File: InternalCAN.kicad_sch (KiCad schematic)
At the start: 7 parts, among them J11 CAN_1, U4 ISO1044BD, U5 CDSOT23-T24CAN

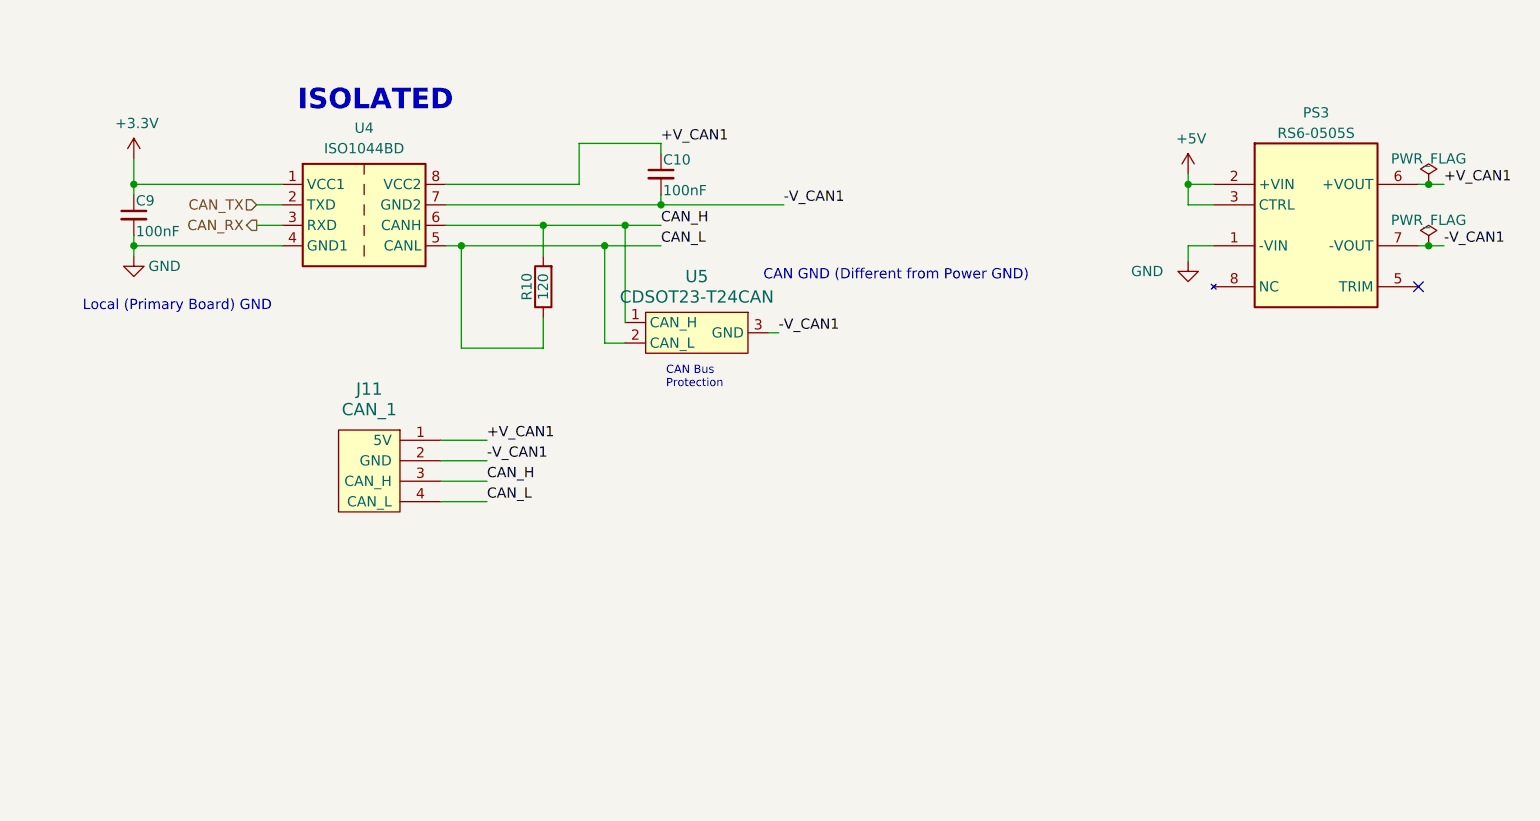
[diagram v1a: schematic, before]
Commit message: a
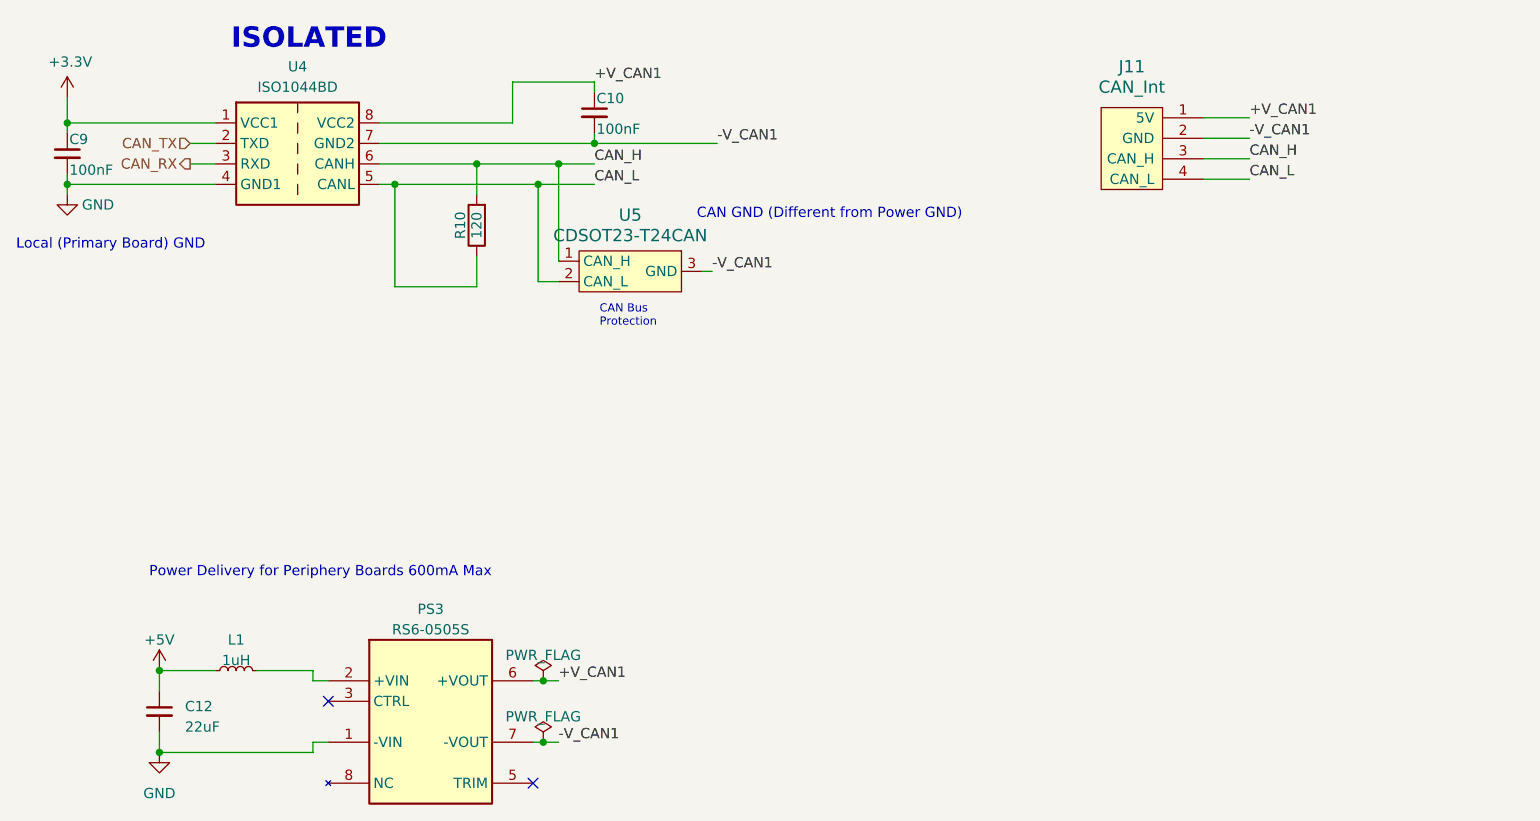
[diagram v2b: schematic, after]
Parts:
- added C12: 22uF, Capacitor_SMD:C_0805_2012Metric, symbol Device:C_Small
- added L1: 1uH, Inductor_SMD:L_0805_2012Metric, symbol Device:L_Small
- J11: value CAN_1 -> CAN_Int
- PS3: footprint RS60505S -> UTSVT_Power:RS60505S
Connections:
- net +5V: now also C12.1, L1.1; no longer PS3.2 (+VIN), PS3.3 (CTRL)
- net GND: now also C12.2
- new net: L1.2, PS3.2 (+VIN)
- no-connect marks 1 -> 2
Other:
- note added: "Power Delivery for Periphery Boards 600mA Max"
- moved on the sheet: C10, C9, J11, PS3, R10, U4, U5

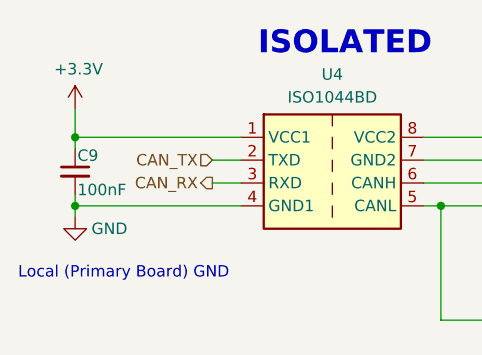
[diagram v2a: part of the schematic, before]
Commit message: updated pin assignments
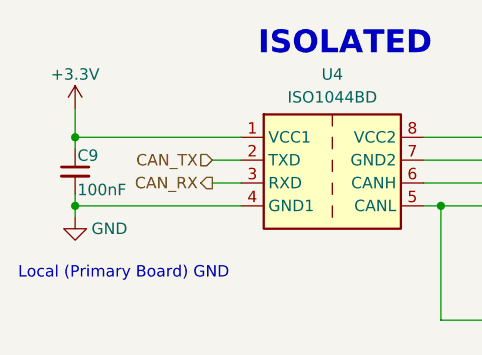
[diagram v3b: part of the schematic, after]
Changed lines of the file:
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@@
     (effects (font (size 1.27 1.27)) (justify right))
-  )
-  (symbol (lib_id "power:+3.3V") (at 75.565 58.42 0) (unit 1)
-    (in_bom yes) (on_board yes) (dnp no)
-    (property "Reference" "#PWR082" (at 75.565 62.23 0)
-      (effects (font (size 1.27 1.27)) hide)
-    )
-    (property "Value" "+3.3V" (at 75.946 54.0258 0)
-      (effects (font (size 1.27 1.27)))
-    )
-    (property "Footprint" "" (at 75.565 58.42 0)
-      (effects (font (size 1.27 1.27)) hide)
-    )
-    (property "Datasheet" "" (at 75.565 58.42 0)
-      (effects (font (size 1.27 1.27)) hide)
-    )
-    (pin "1")
-    (instances
-      (project "LeaderSOM"
-        (path "/192d0c36-944e-4927-949b-263b8c85a7ca/3c3cb7b2-3464-4424-b8df-3064a68eb04d"
-          (reference "#PWR082") (unit 1)
-        )
-      )
-      (project "Dashboard"
-        (path "/66218487-e316-4467-9eba-79d4626ab24e/00000000-0000-0000-0000-00005f547b94"
-          (reference "#PWR0100") (unit 1)
-        )
-      )
-      (project "BPS-PeripheralSOM"
-        (path "/d5ebd247-5a7c-47c2-8aee-beabaef72d6d/1d0c269d-60cf-499b-bfd2-5087981d6678"
-          (reference "#PWR036") (unit 1)
-        )
-      )
-    )
   )
   (symbol (lib_id "power:GND") (at 86.995 139.7 0) (unit 1)
@@
         )
       )
+    )
+  )
+  (symbol (lib_id "power:+3.3V") (at 75.565 58.42 0) (unit 1)
+    (in_bom yes) (on_board yes) (dnp no) (fields_autoplaced)
+    (property "Reference" "#PWR025" (at 75.565 62.23 0)
+      (effects (font (size 1.27 1.27)) hide)
+    )
+    (property "Value" "+3.3V" (at 75.565 54.61 0)
+      (effects (font (size 1.27 1.27)))
+    )
+    (property "Footprint" "" (at 75.565 58.42 0)
+      (effects (font (size 1.27 1.27)) hide)
+    )
+    (property "Datasheet" "" (at 75.565 58.42 0)
+      (effects (font (size 1.27 1.27)) hide)
+    )
+    (pin "1")
+    (instances
+      (project "LeaderSOM"
+        (path "/192d0c36-944e-4927-949b-263b8c85a7ca"
+          (reference "#PWR025") (unit 1)
+        )
+        (path "/192d0c36-944e-4927-949b-263b8c85a7ca/07cef2e6-f2f4-4f04-bcaf-7b98b53ab0fe"
+          (reference "#PWR025") (unit 1)
+        )
+        (path "/192d0c36-944e-4927-949b-263b8c85a7ca/3c3cb7b2-3464-4424-b8df-3064a68eb04d"
+          (reference "#PWR058") (unit 1)
+        )
+      )
+      (project "BPS-PeripheralSOM"
+        (path "/d5ebd247-5a7c-47c2-8aee-beabaef72d6d"
+          (reference "#PWR02") (unit 1)
+        )
+      )
